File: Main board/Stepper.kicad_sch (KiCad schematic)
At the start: 15 parts, among them IC3 DRV8434, J5 Conn_01x04

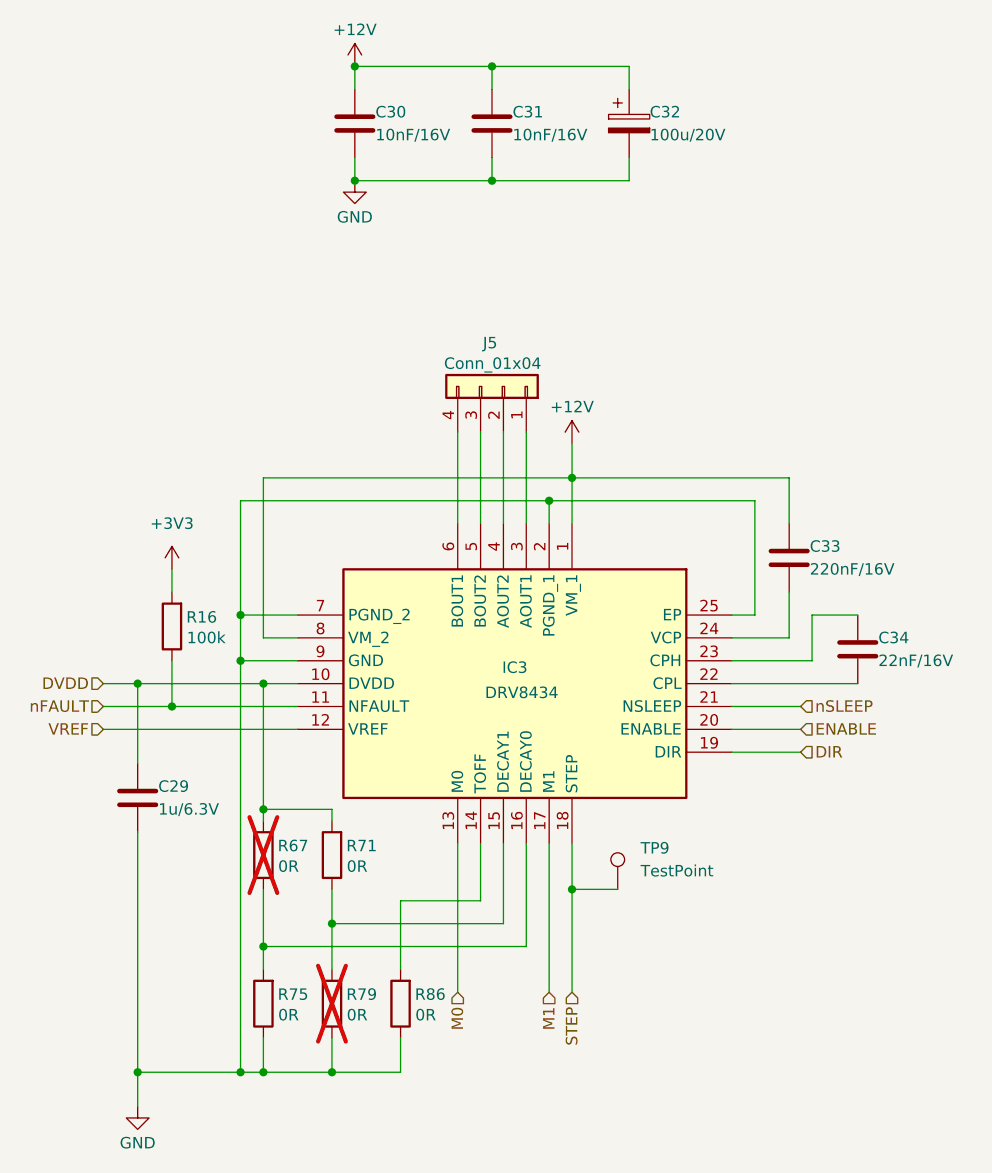
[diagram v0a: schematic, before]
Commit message: schema updated
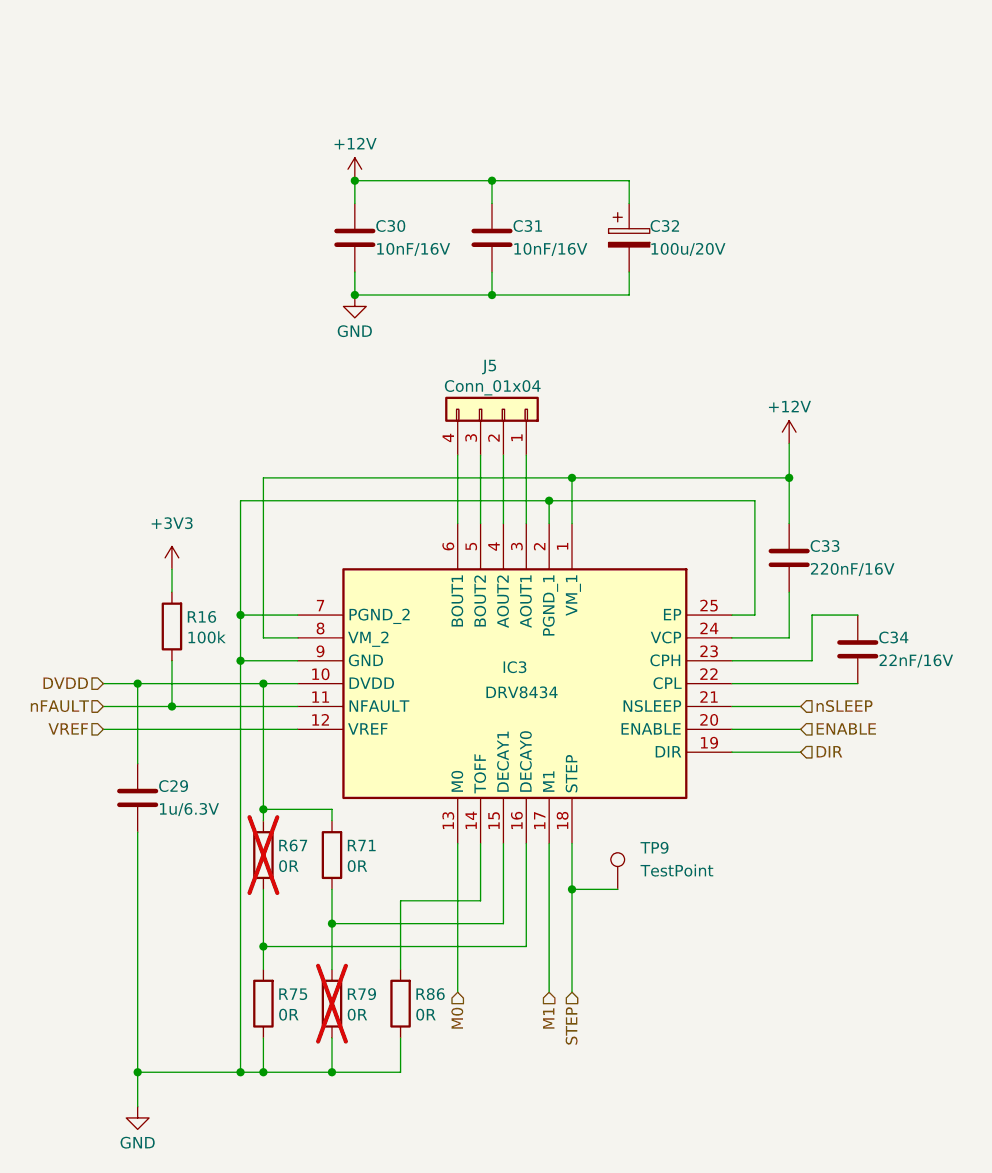
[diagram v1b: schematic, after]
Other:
- moved on the sheet: C30, C31, C32, J5
